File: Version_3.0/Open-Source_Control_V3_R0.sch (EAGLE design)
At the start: 347 parts, among them IC10 MCP6002SMT, IC11 MCP6002SMT, IC12 MCP6002SMT, IC14 MCP6002SMT, IC2 ULN2003AD, IC4 74HC165D, IC5 74HC165D, J24 6p-2.54, K1 G5LE-14-CF DC24, K2 G5LE-14-CF DC24, K3 G5LE-14-CF DC24, K4 G5LE-14-CF DC24, Q1 MMBT2907, T4 DA2304-AL, U1 OSD3358-512M-ICB, U16 AT97SC3205T-G3M4400B, U2 TPD4S012_DRY_6_P1_M, U27 LAN8710, U28 TCAN1051HV, U29 MAX3483EESA+T, U4 APX811-31UGSOT, U40 ISO3086TDW, U5 TLVH431, U6 SN74LVC2G241_DCU_8, X1 10118194-0001LF, X10 MC4, X11 MC4, X12 MC4, X2 J0011D01BNL, X21 MC12, X24 MSTBA2, X3 MC4, X31 MC4, X4 CTI-JTAG, X41 MSTBA3, X5 DM3CS-SF, X6 6p-2.54, X7 TH-2X10, X8 TH-2X10, X9 5600200420, Y7 ECS-250-12-30-GN-TR

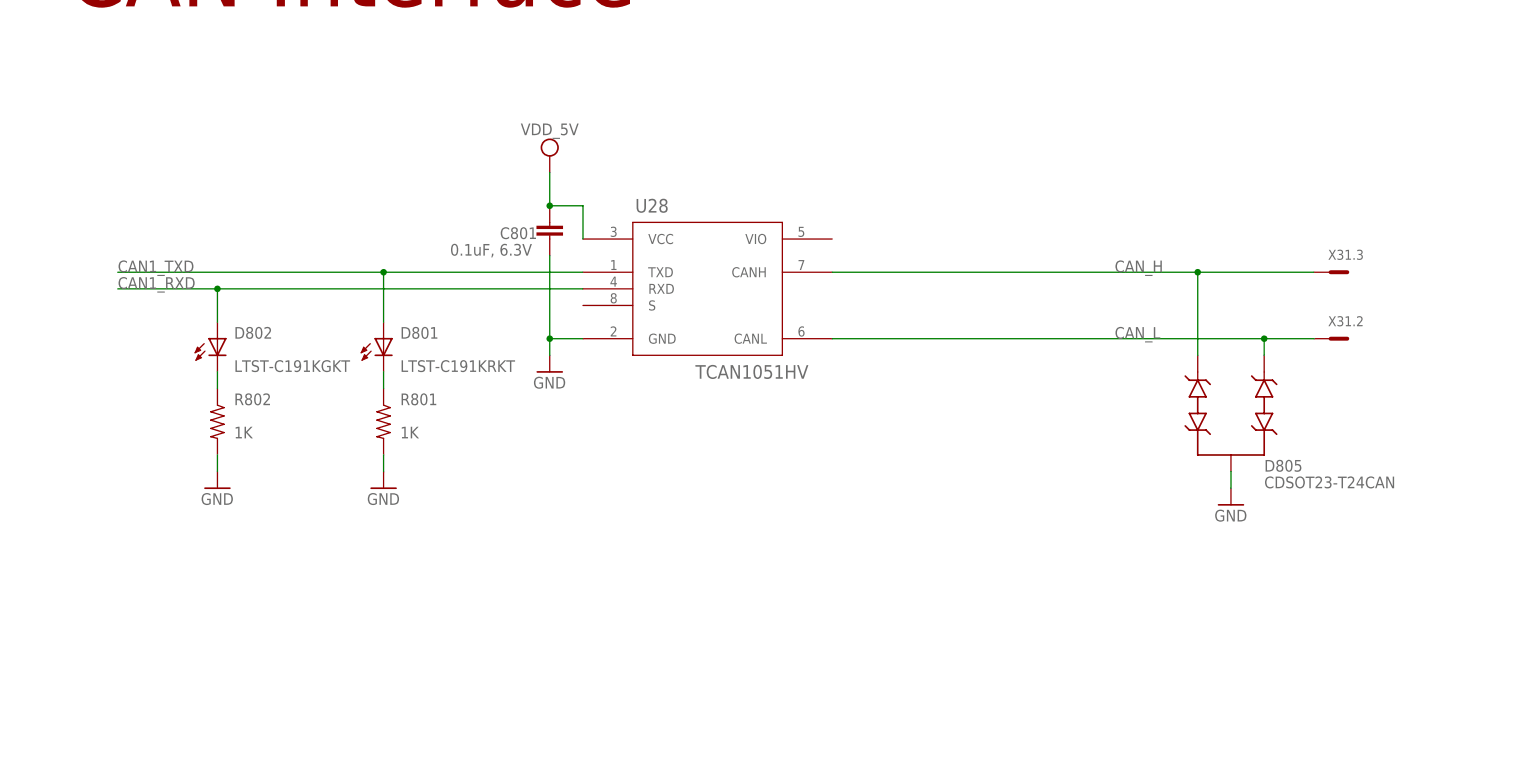
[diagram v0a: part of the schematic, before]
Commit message: Add files via upload
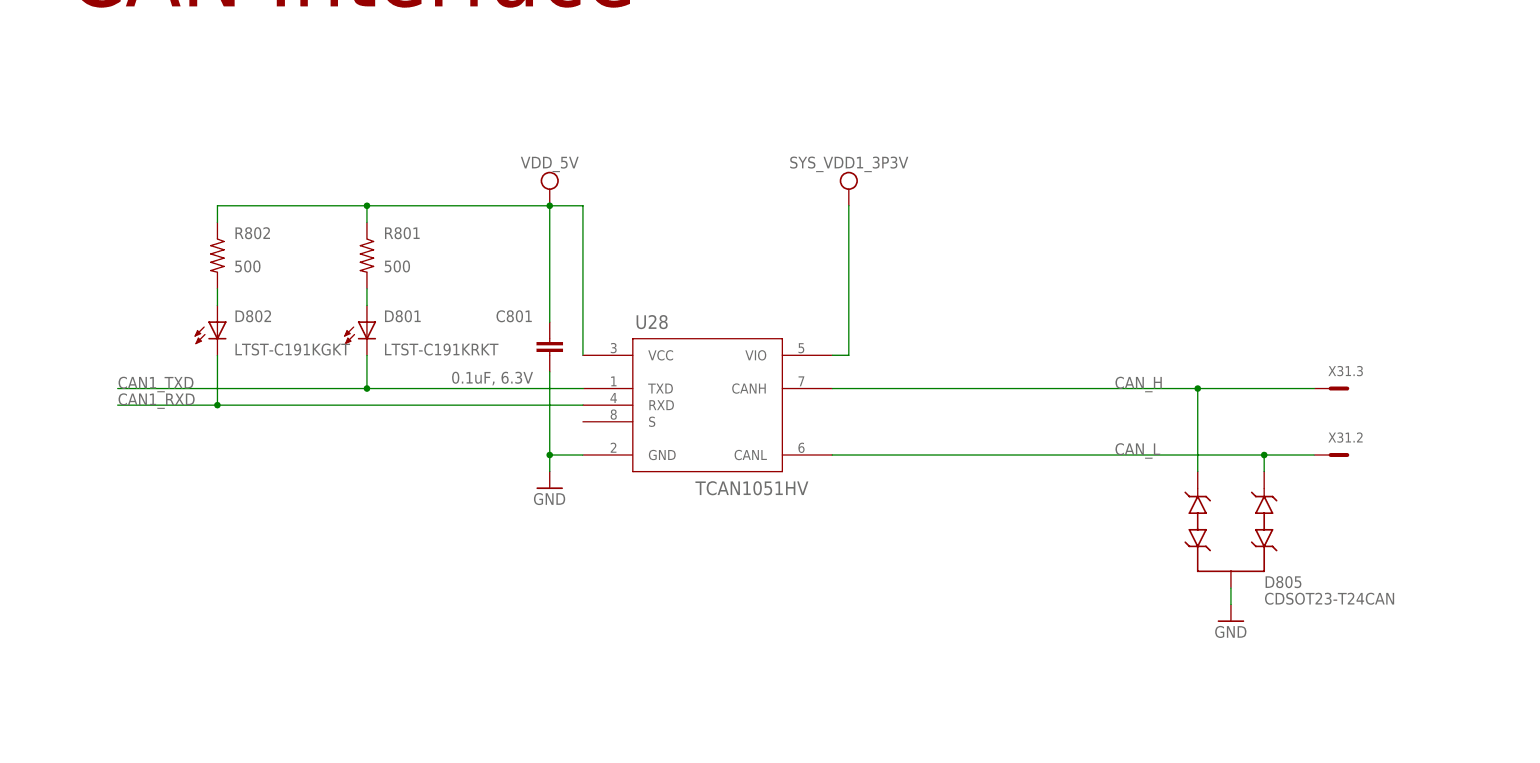
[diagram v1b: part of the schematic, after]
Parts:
- R801, R802: value 1K -> 500
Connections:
- net CAN1_RXD: now also D802.C; no longer D802.A
- net CAN1_TXD: now also D801.C; no longer D801.A
- net GND: no longer R801.2, R802.2
- net N$5: now also D802.A, R802.2; no longer D802.C, R802.1
- net N$6: now also D801.A, R801.2; no longer D801.C, R801.1
- net SYS_VDD1_3P3V: now also U28.VIO
- net VDD_5V: now also R801.1, R802.1
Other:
- moved on the sheet: C801, D801, D802, D805, R801, R802, U28, X31.2, X31.3

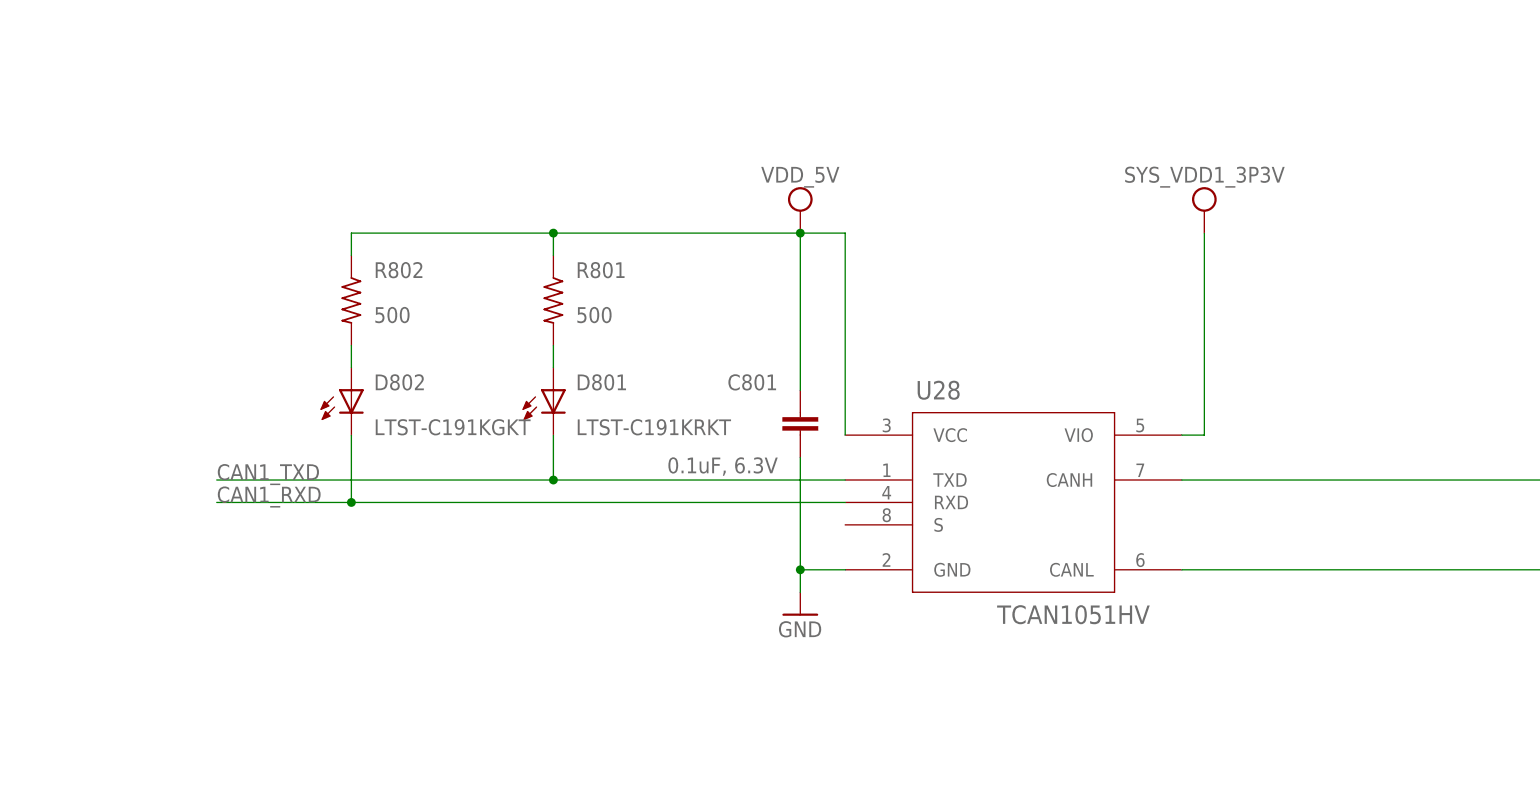
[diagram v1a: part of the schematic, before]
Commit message: Add files via upload
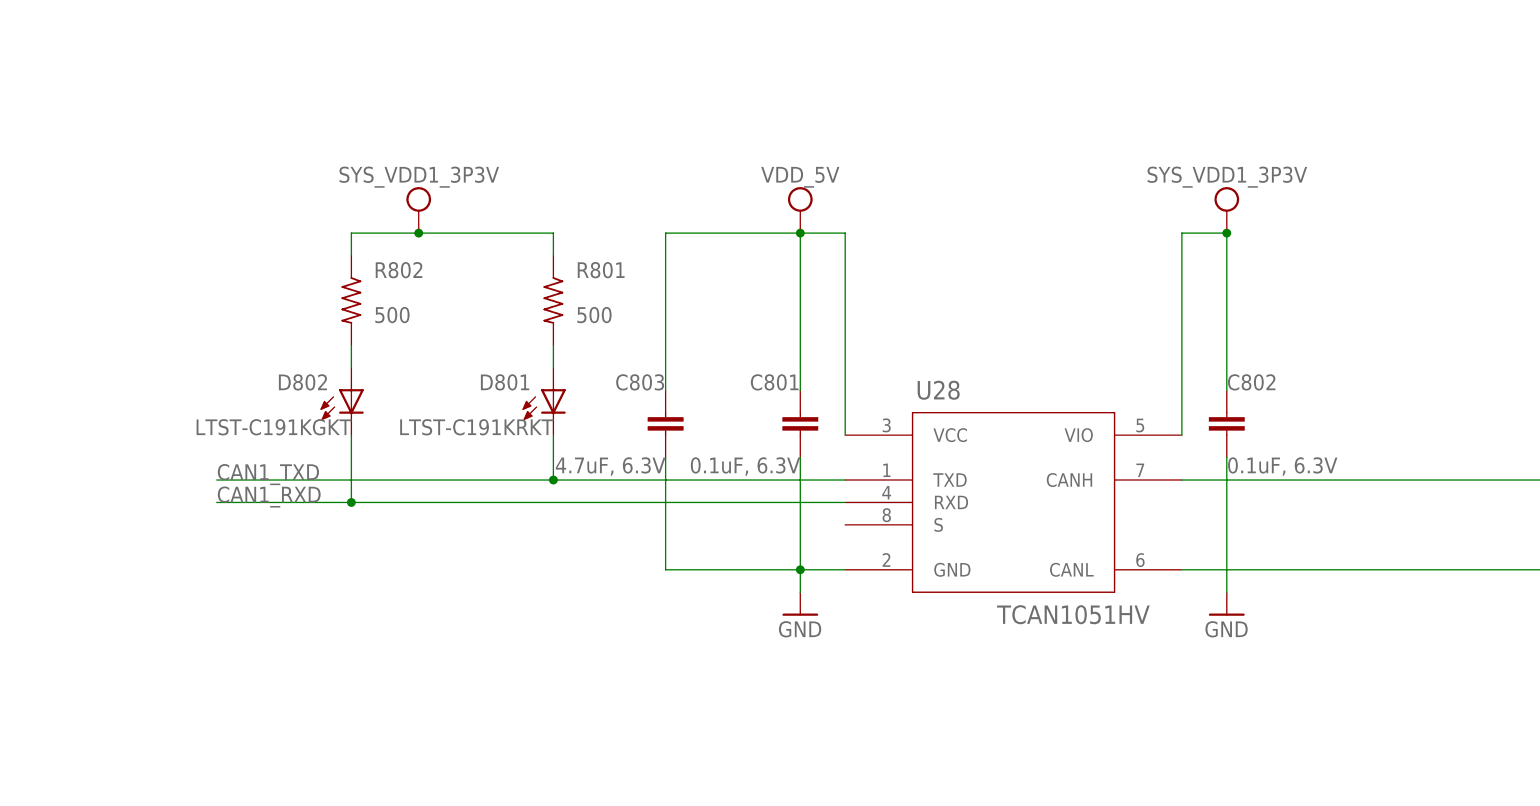
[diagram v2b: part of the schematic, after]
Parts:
- added C802: 0.1uF, 6.3V, OSD3358-SM-RED Platform:CC0402
- added C803: 4.7uF, 6.3V, OSD3358-SM-RED Platform:CC0402
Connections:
- net GND: now also C802.2, C803.2
- net SYS_VDD1_3P3V: now also C802.1, R801.1, R802.1
- net VDD_5V: now also C803.1; no longer R801.1, R802.1
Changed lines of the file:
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@@
 <part name="SUPPLY36" library="OSD3358-SM-RED Platform" deviceset="VDD_5V" device=""/>
 <part name="SUPPLY37" library="OSD3358-SM-RED Platform" deviceset="SYS_VDD1_3P3V" device=""/>
+<part name="C802" library="OSD3358-SM-RED Platform" deviceset="C" device="C0402" value="0.1uF, 6.3V"/>
+<part name="GND1" library="OSD3358-SM-RED Platform" deviceset="GND" device=""/>
+<part name="SUPPLY39" library="OSD3358-SM-RED Platform" deviceset="SYS_VDD1_3P3V" device=""/>
+<part name="C803" library="OSD3358-SM-RED Platform" deviceset="C" device="C0402" value="4.7uF, 6.3V"/>
 </parts>
 <sheets>
@@
 </instance>
 <instance part="D801" gate="G$1" x="853.44" y="685.8" smashed="yes">
-<attribute name="NAME" x="855.98" y="685.8" size="1.778" layer="95"/>
-<attribute name="VALUE" x="855.98" y="680.72" size="1.778" layer="96"/>
+<attribute name="NAME" x="850.9" y="685.8" size="1.778" layer="95" align="bottom-right"/>
+<attribute name="VALUE" x="853.44" y="680.72" size="1.778" layer="96" align="bottom-right"/>
 </instance>
 <instance part="D802" gate="G$1" x="830.58" y="685.8" smashed="yes">
-<attribute name="NAME" x="833.12" y="685.8" size="1.778" layer="95"/>
-<attribute name="VALUE" x="833.12" y="680.72" size="1.778" layer="96"/>
+<attribute name="NAME" x="828.04" y="685.8" size="1.778" layer="95" align="bottom-right"/>
+<attribute name="VALUE" x="830.58" y="680.72" size="1.778" layer="96" align="bottom-right"/>
 </instance>
 <instance part="R802" gate="G$1" x="830.58" y="695.96" smashed="yes" rot="R270">
@@
 </instance>
 <instance part="C801" gate="G$1" x="881.38" y="683.26" smashed="yes">
-<attribute name="NAME" x="878.84" y="685.8" size="1.778" layer="95" align="bottom-right"/>
-<attribute name="VALUE" x="878.84" y="678.18" size="1.778" layer="96" align="top-right"/>
+<attribute name="NAME" x="881.38" y="685.8" size="1.778" layer="95" align="bottom-right"/>
+<attribute name="VALUE" x="881.38" y="678.18" size="1.778" layer="96" align="top-right"/>
 </instance>
 <instance part="R303" gate="G$1" x="962.66" y="812.8" smashed="yes" rot="R90">
@@
 <attribute name="VALUE" x="881.38" y="710.184" size="1.778" layer="96" align="center"/>
 </instance>
-<instance part="SUPPLY37" gate="G$1" x="927.1" y="706.12" smashed="yes">
-<attribute name="VALUE" x="927.1" y="710.184" size="1.778" layer="96" align="center"/>
+<instance part="SUPPLY37" gate="G$1" x="929.64" y="706.12" smashed="yes">
+<attribute name="VALUE" x="929.64" y="710.184" size="1.778" layer="96" align="center"/>
+</instance>
+<instance part="C802" gate="G$1" x="929.64" y="683.26" smashed="yes">
+<attribute name="NAME" x="929.64" y="685.8" size="1.778" layer="95"/>
+<attribute name="VALUE" x="929.64" y="678.18" size="1.778" layer="96" align="top-left"/>
+</instance>
+<instance part="GND1" gate="1" x="929.64" y="660.4" smashed="yes">
+<attribute name="VALUE" x="927.1" y="657.86" size="1.778" layer="96"/>
+</instance>
+<instance part="SUPPLY39" gate="G$1" x="838.2" y="706.12" smashed="yes">
+<attribute name="VALUE" x="838.2" y="710.184" size="1.778" layer="96" align="center"/>
+</instance>
+<instance part="C803" gate="G$1" x="866.14" y="683.26" smashed="yes">
+<attribute name="NAME" x="866.14" y="685.8" size="1.778" layer="95" align="bottom-right"/>
+<attribute name="VALUE" x="866.14" y="678.18" size="1.778" layer="96" align="top-right"/>
 </instance>
 </instances>
@@
 <segment>
 <pinref part="SUPPLY36" gate="G$1" pin="VDD_5V"/>
-<pinref part="R802" gate="G$1" pin="1"/>
-<wire x1="881.38" y1="703.58" x2="853.44" y2="703.58" width="0.1524" layer="91"/>
-<wire x1="853.44" y1="703.58" x2="830.58" y2="703.58" width="0.1524" layer="91"/>
-<wire x1="830.58" y1="703.58" x2="830.58" y2="701.04" width="0.1524" layer="91"/>
-<pinref part="R801" gate="G$1" pin="1"/>
-<wire x1="853.44" y1="701.04" x2="853.44" y2="703.58" width="0.1524" layer="91"/>
-<junction x="853.44" y="703.58"/>
 <pinref part="C801" gate="G$1" pin="1"/>
 <wire x1="881.38" y1="703.58" x2="881.38" y2="685.8" width="0.1524" layer="91"/>
@@
 <wire x1="886.46" y1="680.72" x2="886.46" y2="703.58" width="0.1524" layer="91"/>
 <wire x1="886.46" y1="703.58" x2="881.38" y2="703.58" width="0.1524" layer="91"/>
+<wire x1="881.38" y1="703.58" x2="866.14" y2="703.58" width="0.1524" layer="91"/>
+<pinref part="C803" gate="G$1" pin="1"/>
+<wire x1="866.14" y1="703.58" x2="866.14" y2="685.8" width="0.1524" layer="91"/>
 </segment>
 </net>
@@
 <wire x1="881.38" y1="678.18" x2="881.38" y2="665.48" width="0.1524" layer="91"/>
 <junction x="881.38" y="665.48"/>
+<pinref part="C803" gate="G$1" pin="2"/>
+<wire x1="866.14" y1="678.18" x2="866.14" y2="665.48" width="0.1524" layer="91"/>
+<wire x1="866.14" y1="665.48" x2="881.38" y2="665.48" width="0.1524" layer="91"/>
 </segment>
 <segment>
@@
 <junction x="1145.54" y="772.16"/>
 </segment>
+<segment>
+<pinref part="C802" gate="G$1" pin="2"/>
+<pinref part="GND1" gate="1" pin="GND"/>
+<wire x1="929.64" y1="678.18" x2="929.64" y2="662.94" width="0.1524" layer="91"/>
+</segment>
 </net>
 <net name="PWR_BUT" class="0">
@@
 <pinref part="U28" gate="G$1" pin="VIO"/>
 <pinref part="SUPPLY37" gate="G$1" pin="SYS_VDD1_3P3V"/>
-<wire x1="924.56" y1="680.72" x2="927.1" y2="680.72" width="0.1524" layer="91"/>
-<wire x1="927.1" y1="680.72" x2="927.1" y2="703.58" width="0.1524" layer="91"/>
+<wire x1="924.56" y1="680.72" x2="924.56" y2="703.58" width="0.1524" layer="91"/>
+<wire x1="924.56" y1="703.58" x2="929.64" y2="703.58" width="0.1524" layer="91"/>
+<pinref part="C802" gate="G$1" pin="1"/>
+<wire x1="929.64" y1="685.8" x2="929.64" y2="703.58" width="0.1524" layer="91"/>
+<junction x="929.64" y="703.58"/>
+</segment>
+<segment>
+<pinref part="SUPPLY39" gate="G$1" pin="SYS_VDD1_3P3V"/>
+<pinref part="R802" gate="G$1" pin="1"/>
+<wire x1="838.2" y1="703.58" x2="830.58" y2="703.58" width="0.1524" layer="91"/>
+<wire x1="830.58" y1="703.58" x2="830.58" y2="701.04" width="0.1524" layer="91"/>
+<pinref part="R801" gate="G$1" pin="1"/>
+<wire x1="853.44" y1="701.04" x2="853.44" y2="703.58" width="0.1524" layer="91"/>
+<wire x1="853.44" y1="703.58" x2="838.2" y2="703.58" width="0.1524" layer="91"/>
+<junction x="838.2" y="703.58"/>
 </segment>
 </net>
